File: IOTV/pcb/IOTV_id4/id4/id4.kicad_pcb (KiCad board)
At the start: 2 copper layers, 109.2 x 73.7 mm, 57 parts, among them Q1 S8050, Q10 S8050, Q11 S8050, Q12 S8050, Q13 S8050, Q14 S8050, Q15 S8050, Q2 S8050, Q3 S8050, Q4 S8050, Q5 S8050, Q6 S8050, Q7 S8050, Q8 S8050, Q9 S8050, SW1 SW_Push, SW2 SW_Push, SW3 SW_Push, U1 ESP32_DevKit_V1_DOIT, U2 DFR0299

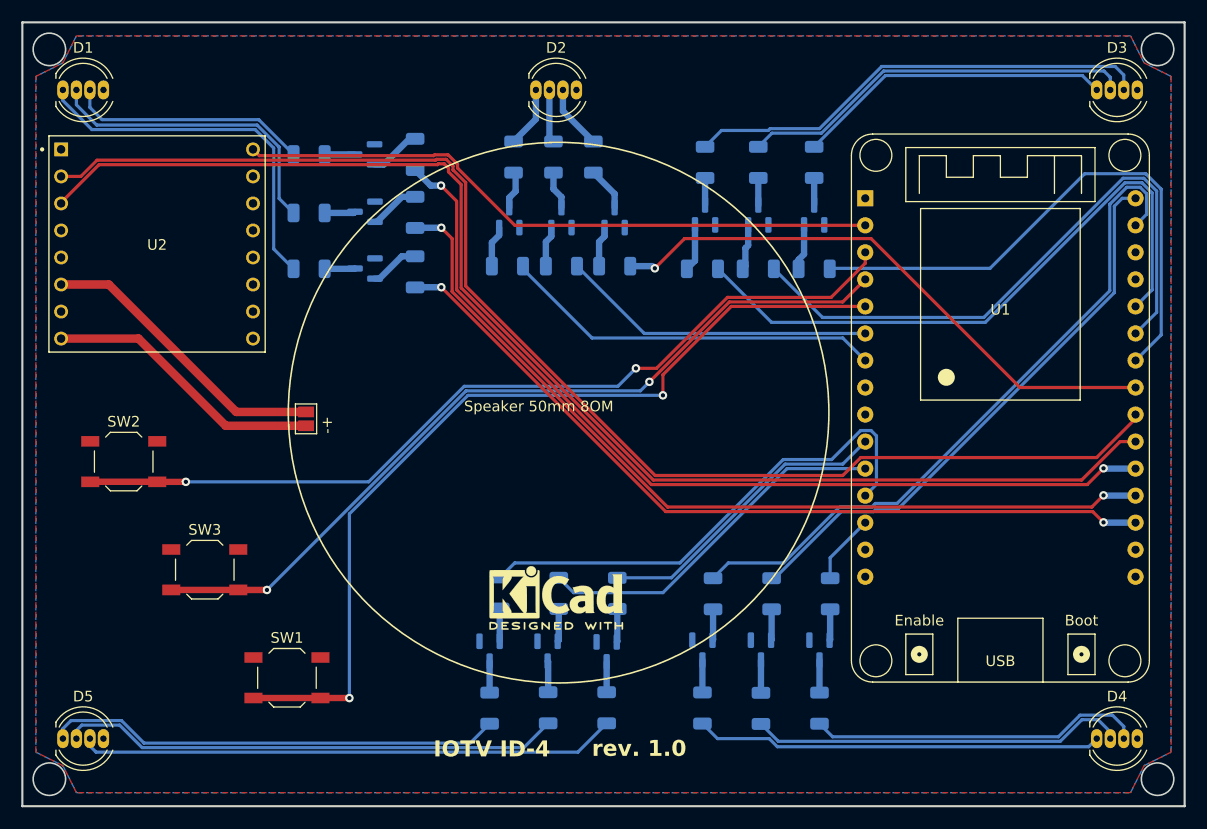
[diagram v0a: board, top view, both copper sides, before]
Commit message: pcb id4
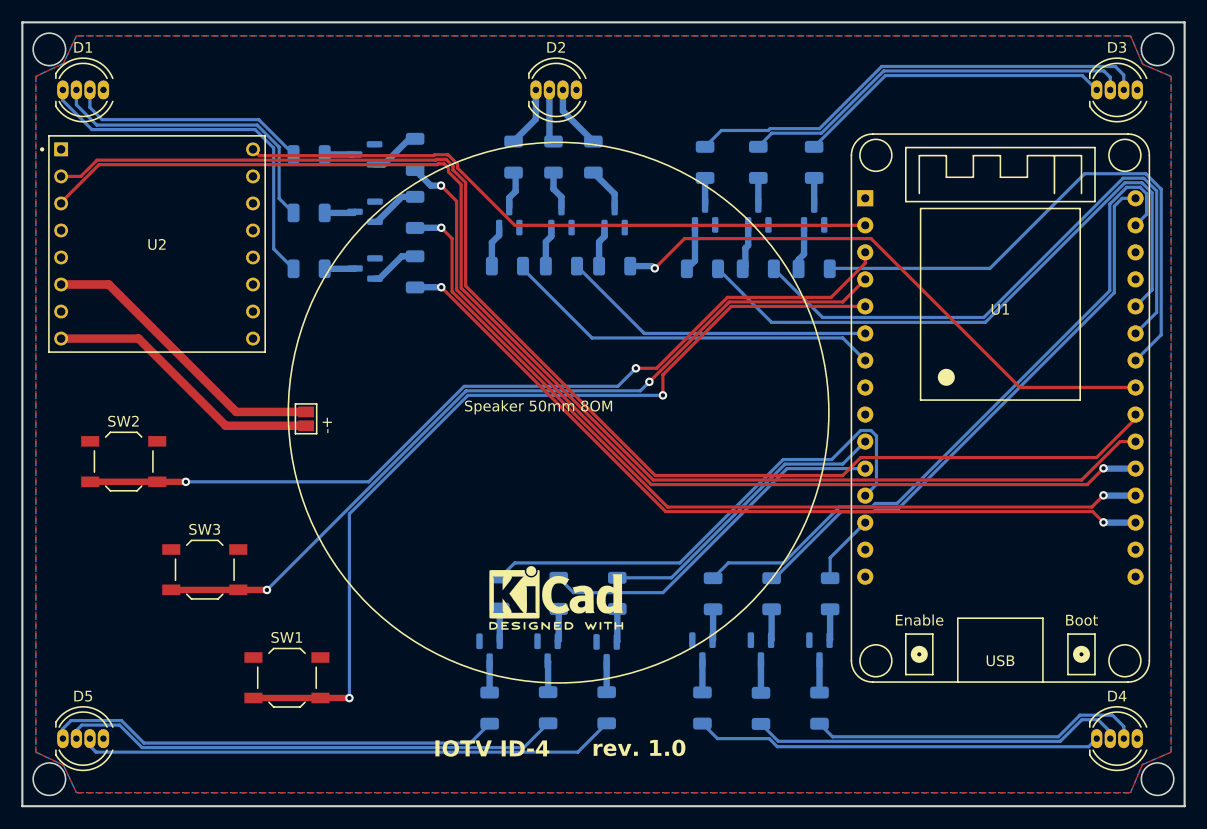
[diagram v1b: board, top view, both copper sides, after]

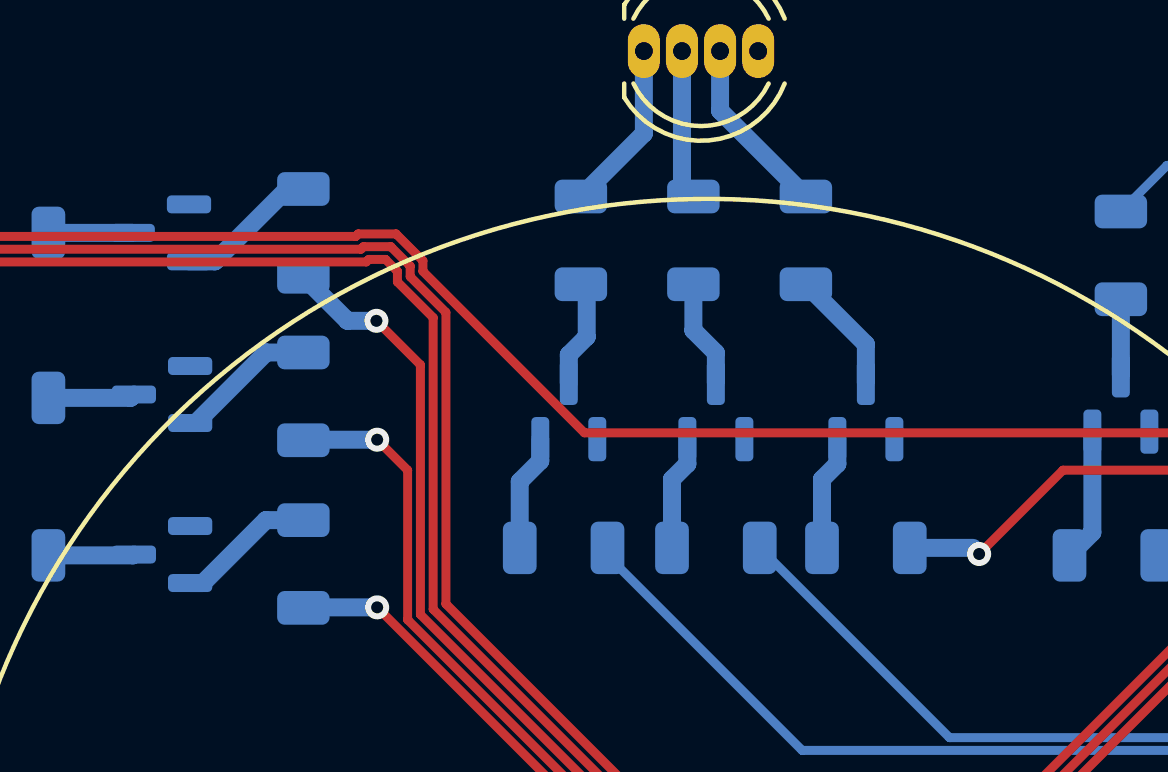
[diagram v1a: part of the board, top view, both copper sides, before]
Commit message: id4 cad
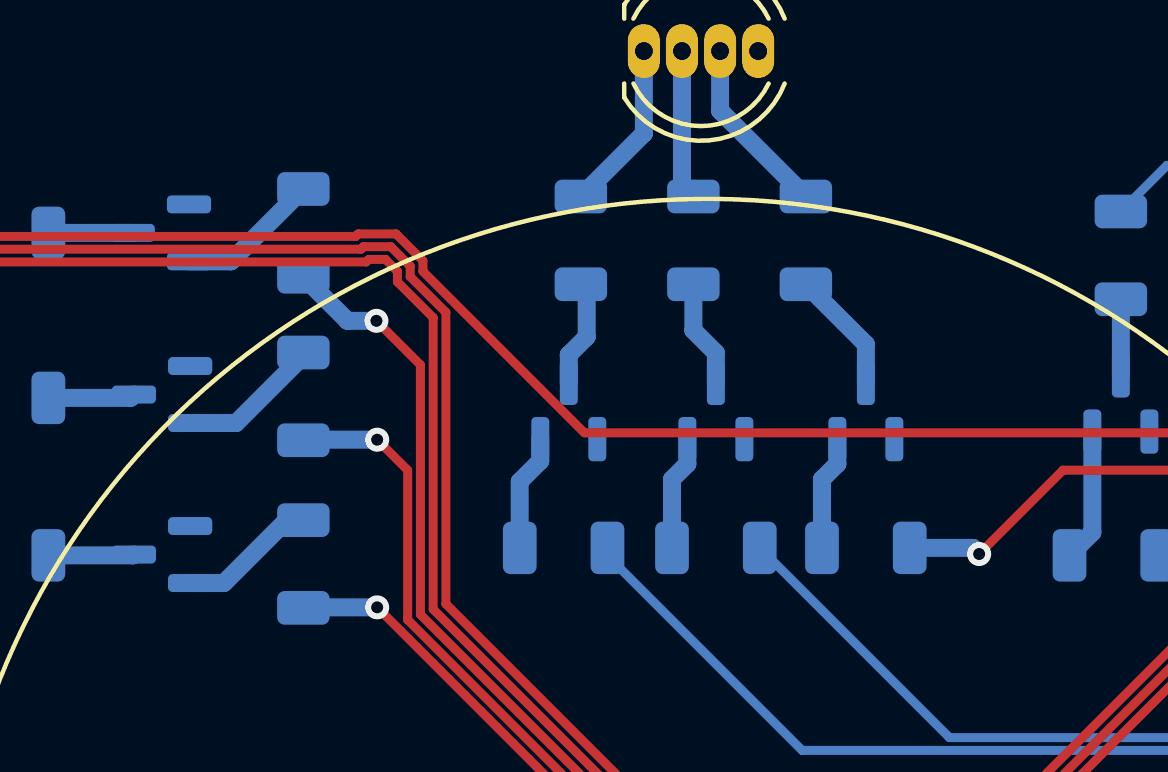
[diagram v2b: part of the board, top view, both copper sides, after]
